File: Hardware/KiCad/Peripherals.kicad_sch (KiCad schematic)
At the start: 71 parts

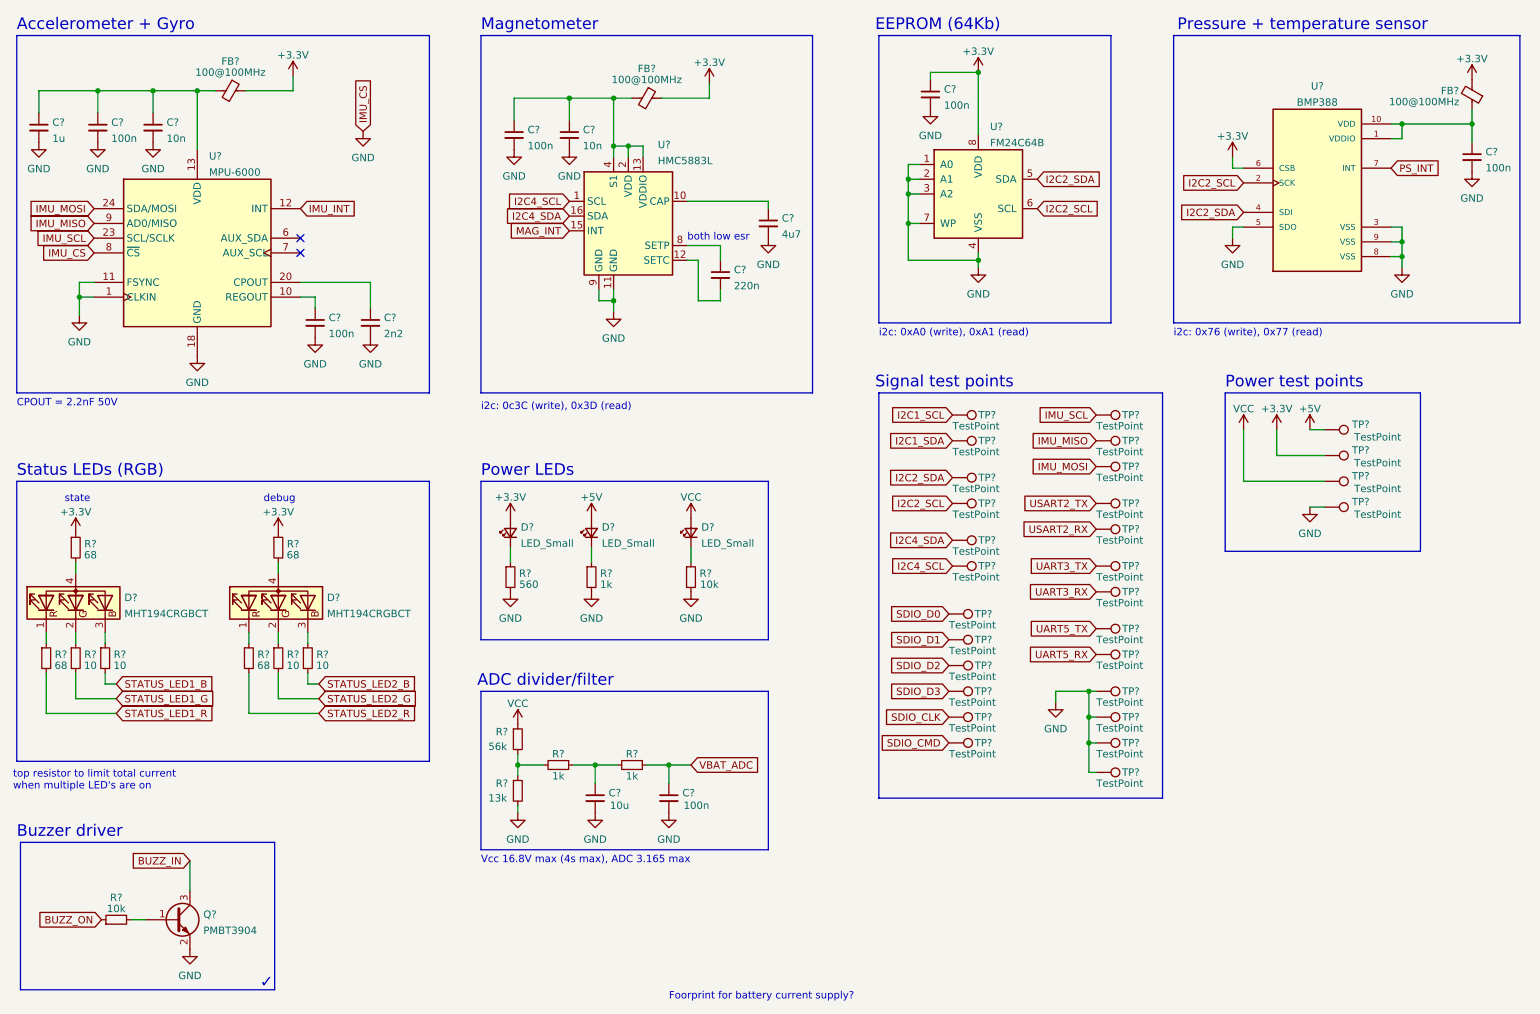
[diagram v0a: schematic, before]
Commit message: Final schematic changes made, added some annotations
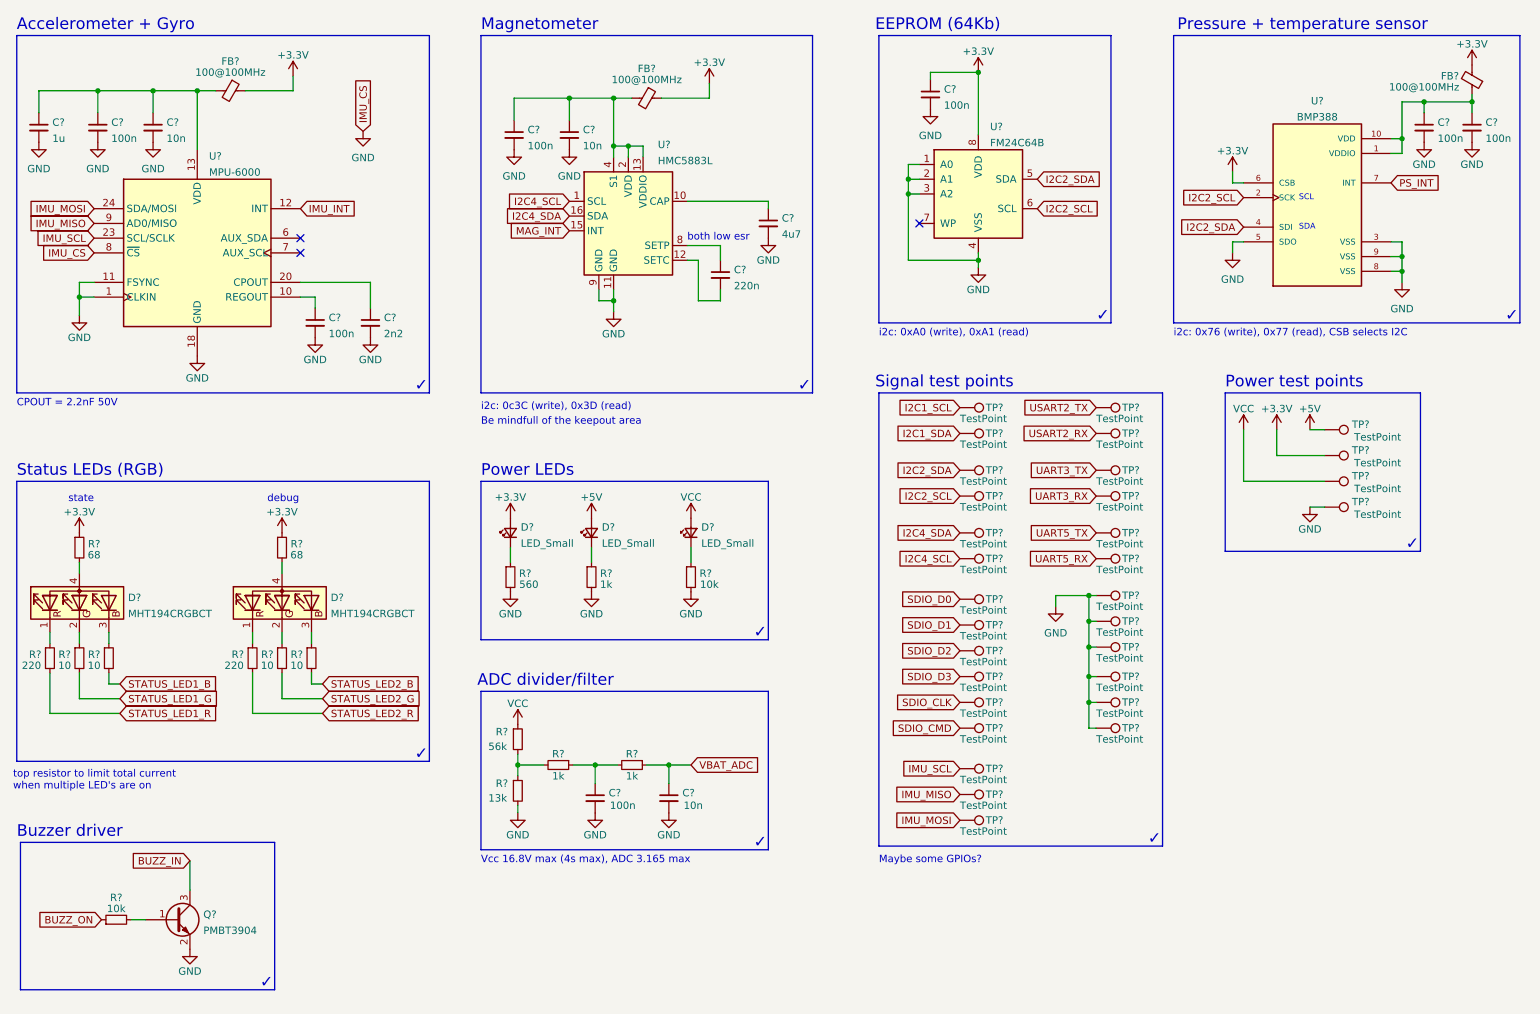
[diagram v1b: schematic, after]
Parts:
- removed C?: 10u, Capacitor_SMD:C_0603_1608Metric, symbol Device:C_Small
- added C? (x2): 100n, Capacitor_SMD:C_0402_1005Metric, symbol Device:C_Small
- added TP? (x2): TestPoint, TestPoint:TestPoint_Pad_D1.5mm, symbol Connector:TestPoint
- C?: value 100n -> 10n
- R? (x2): value 68 -> 220
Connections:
- net GND: now also C?.2, C?.2, TP?.1, TP?.1; no longer U?.7 (WP)
- net at C?.1, FB?.1, U?.1 (VDDIO)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: now also C?.1
- net at R?.1, R?.2: now also C?.1
- no-connect marks 2 -> 3
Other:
- note added: "Be mindfull of the keepout area"
- note added: "Maybe some GPIOs?"
- note added: "SCL"
- note added: "SDA"
- note added: "i2c: 0x76 (write), 0x77 (read), CSB selects I2C"
- note removed: "Foorprint for battery current supply?"
- note removed: "i2c: 0x76 (write), 0x77 (read)"
- moved on the sheet: C?, D?, FB?, R?, TP?, U?
